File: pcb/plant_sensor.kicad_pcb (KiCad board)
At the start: 2 copper layers, 21 parts, among them IC1 SPBTLE-RF0, IC2 STM32L052K8Tx, J1 Conn_ARM_JTAG_SWD_10, J2 COM, U1 M95256-WMN6P, Y1 32.768kHz

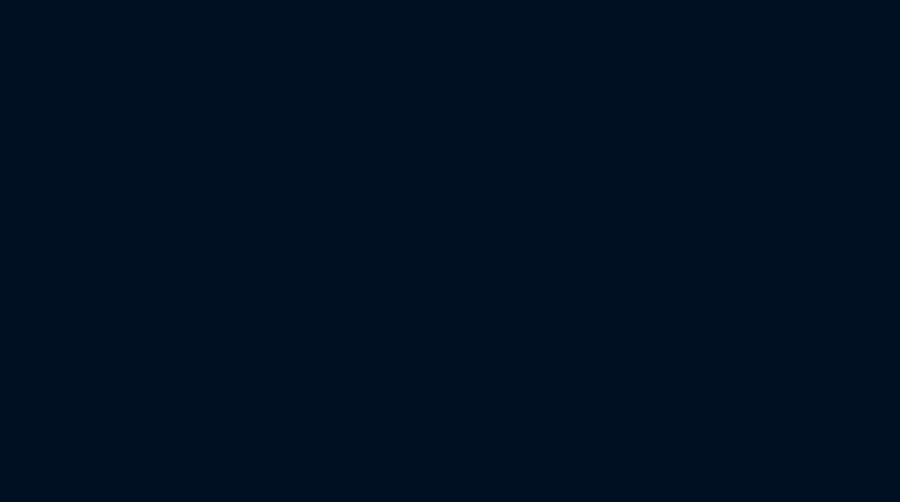
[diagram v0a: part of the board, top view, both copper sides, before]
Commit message: Added temperature sensor
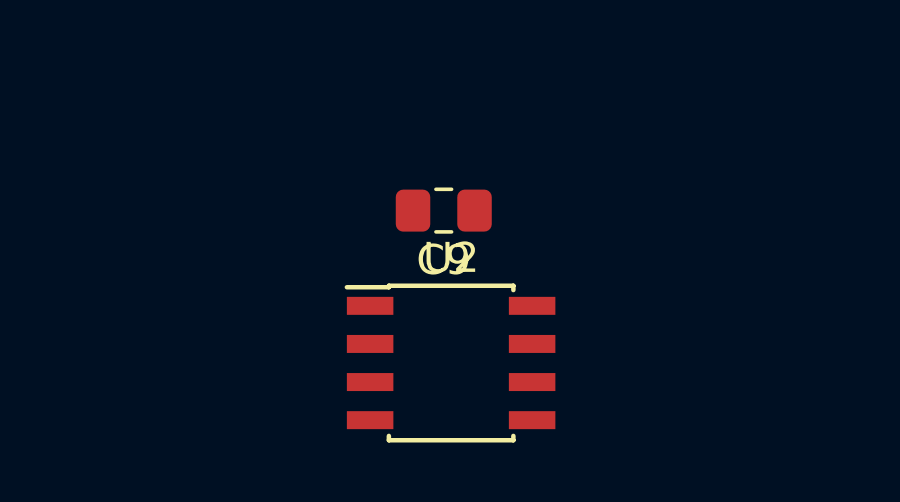
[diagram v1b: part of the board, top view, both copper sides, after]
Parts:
- added C9: 100nF, Capacitor_SMD:C_0805_2012Metric_Pad1.15x1.40mm_HandSolder, F.Cu at (98.8, 96.5)
- added U2: LM75B, Package_SO:SOIC-8_3.9x4.9mm_P1.27mm, F.Cu at (99.1, 101.6)
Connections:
- net Net-(R5-Pad1) renamed /MCU/LED
- IC2 pad 28: Net-(IC2-Pad28) -> /MCU/TEMP_IRQ
- IC2 pad 29: Net-(IC2-Pad29) -> /MCU/I2C1_SCL
- IC2 pad 30: Net-(IC2-Pad30) -> /MCU/I2C1_SDA
